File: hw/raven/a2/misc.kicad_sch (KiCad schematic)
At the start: 62 parts, among them J601 TRSx2, J602 PinHdr_01x04, J603 PinHdr_01x04, J604 PinHdr_01x04, J605 DB25/9/9, J606 DB9M/9M, J607 USB+Ethernet, J608 PinHdr_01x04, U601 CNY17F-3, U602 74LS07

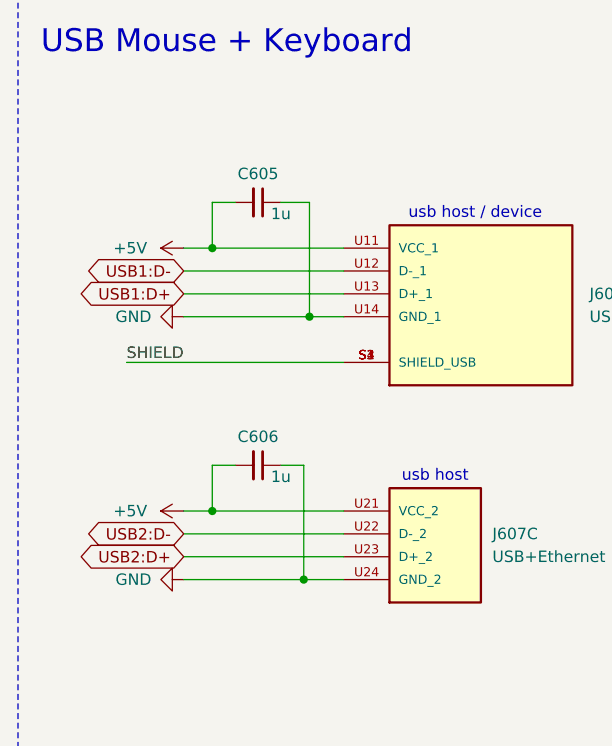
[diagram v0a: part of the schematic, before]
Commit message: a2 wip
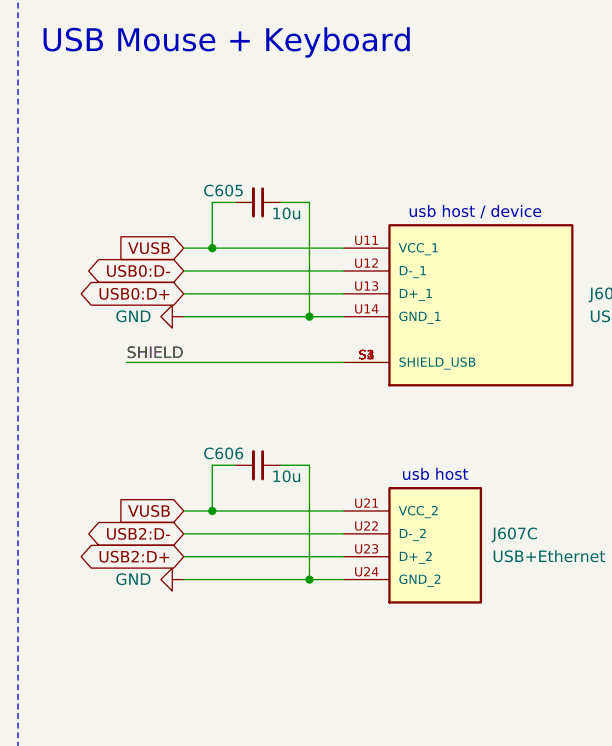
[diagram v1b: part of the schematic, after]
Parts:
- C605, C606: value 1u -> 10u; Manufacturer_Part_Number C1206C105K4RACTU -> C1206C106K4RAC
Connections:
- net +5V: no longer C605.2, C606.2, J607.U11 (VCC_1), J607.U21 (VCC_2)
- net USB1:D+ renamed USB0:D+
- net USB1:D- renamed USB0:D-
- new net VUSB: C605.2, C606.2, J607.U11 (VCC_1), J607.U21 (VCC_2)
